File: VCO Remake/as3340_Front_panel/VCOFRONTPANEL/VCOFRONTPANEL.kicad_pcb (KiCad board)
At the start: 2 copper layers, 20.3 x 128.5 mm, 19 parts

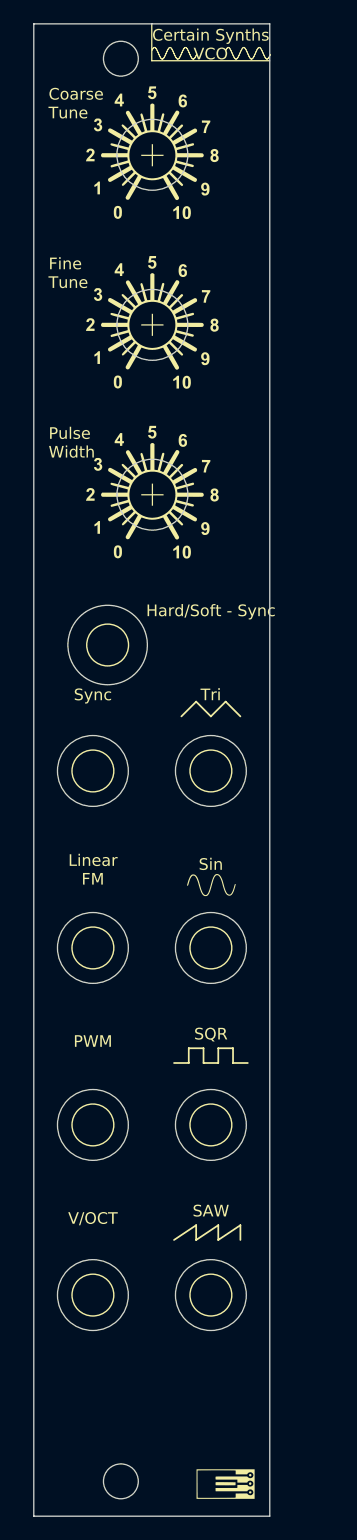
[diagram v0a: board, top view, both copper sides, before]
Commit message: e
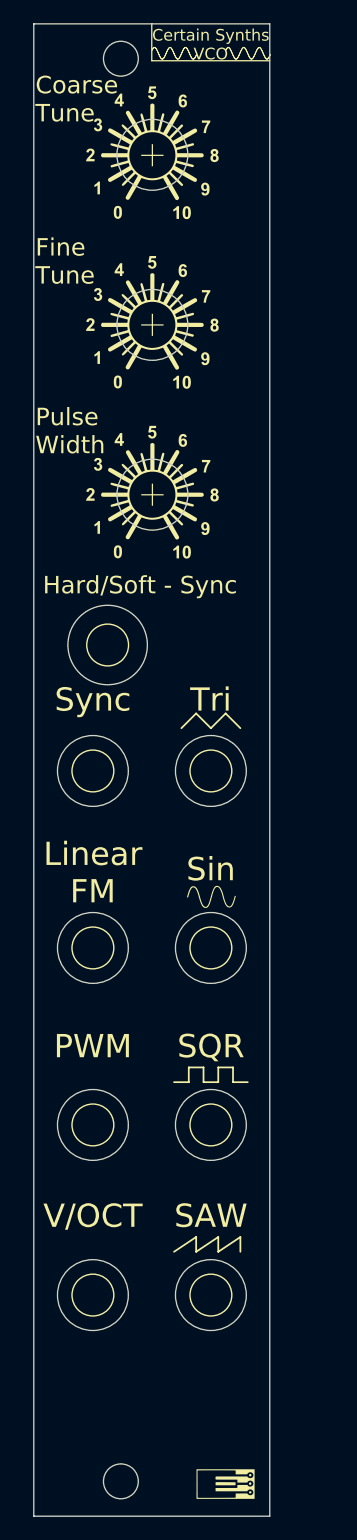
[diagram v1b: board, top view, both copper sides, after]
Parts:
- moved G*** 1.02 mm to (154.2, 108.0)
